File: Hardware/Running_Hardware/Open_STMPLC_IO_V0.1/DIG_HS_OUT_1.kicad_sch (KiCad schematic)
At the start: 25 parts, among them J1 Screw_Terminal_01x02, Q1 SUD50P06, Q2 AO3400A, U7 TPS26600PWP, U8 UCC23513

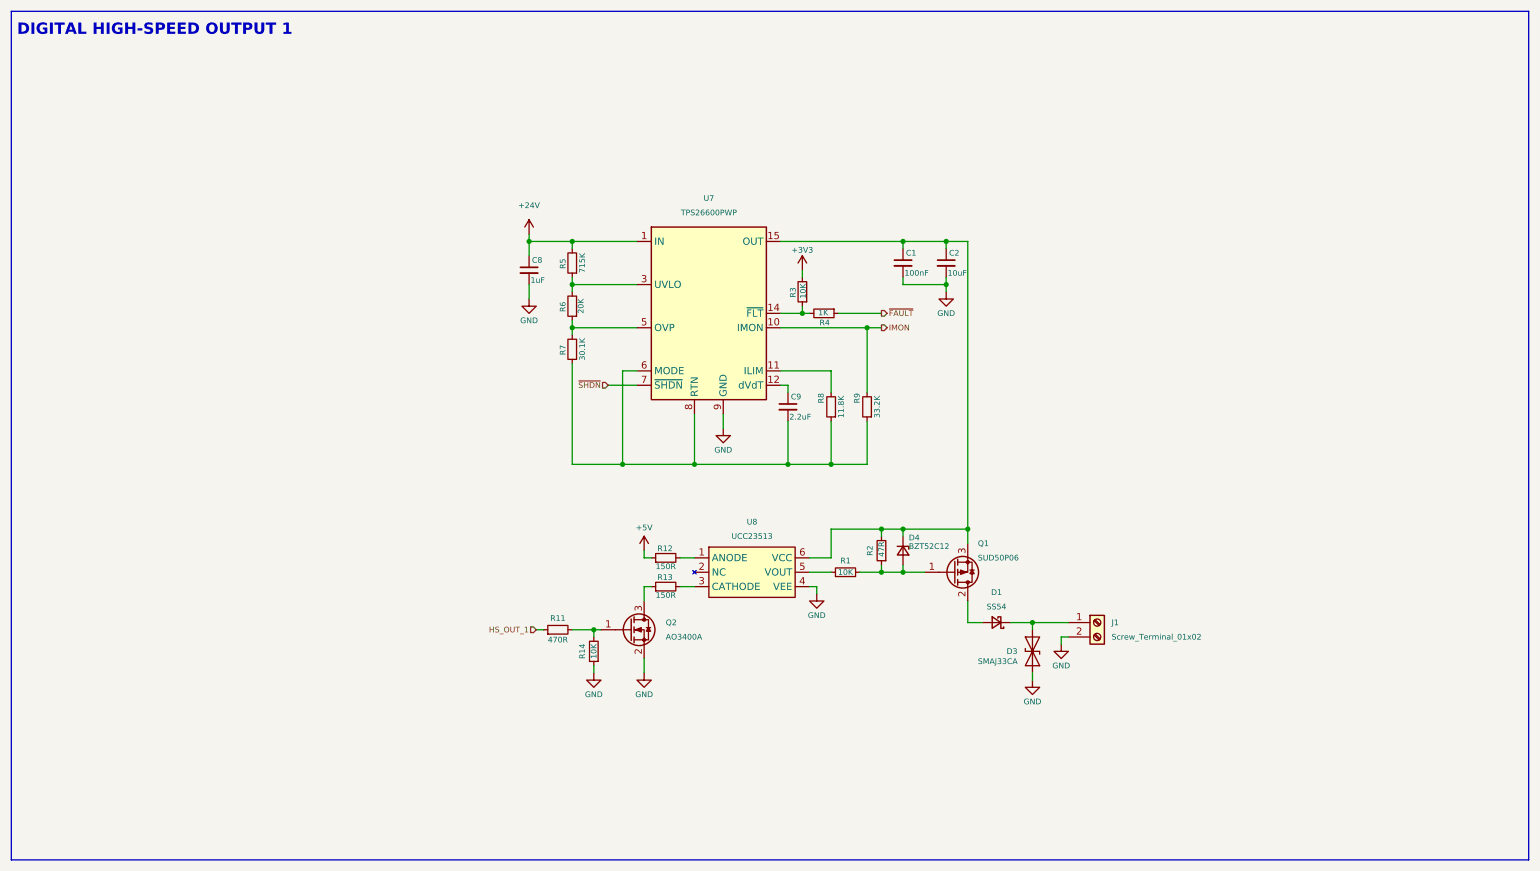
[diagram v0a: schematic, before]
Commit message: Digital IO completion
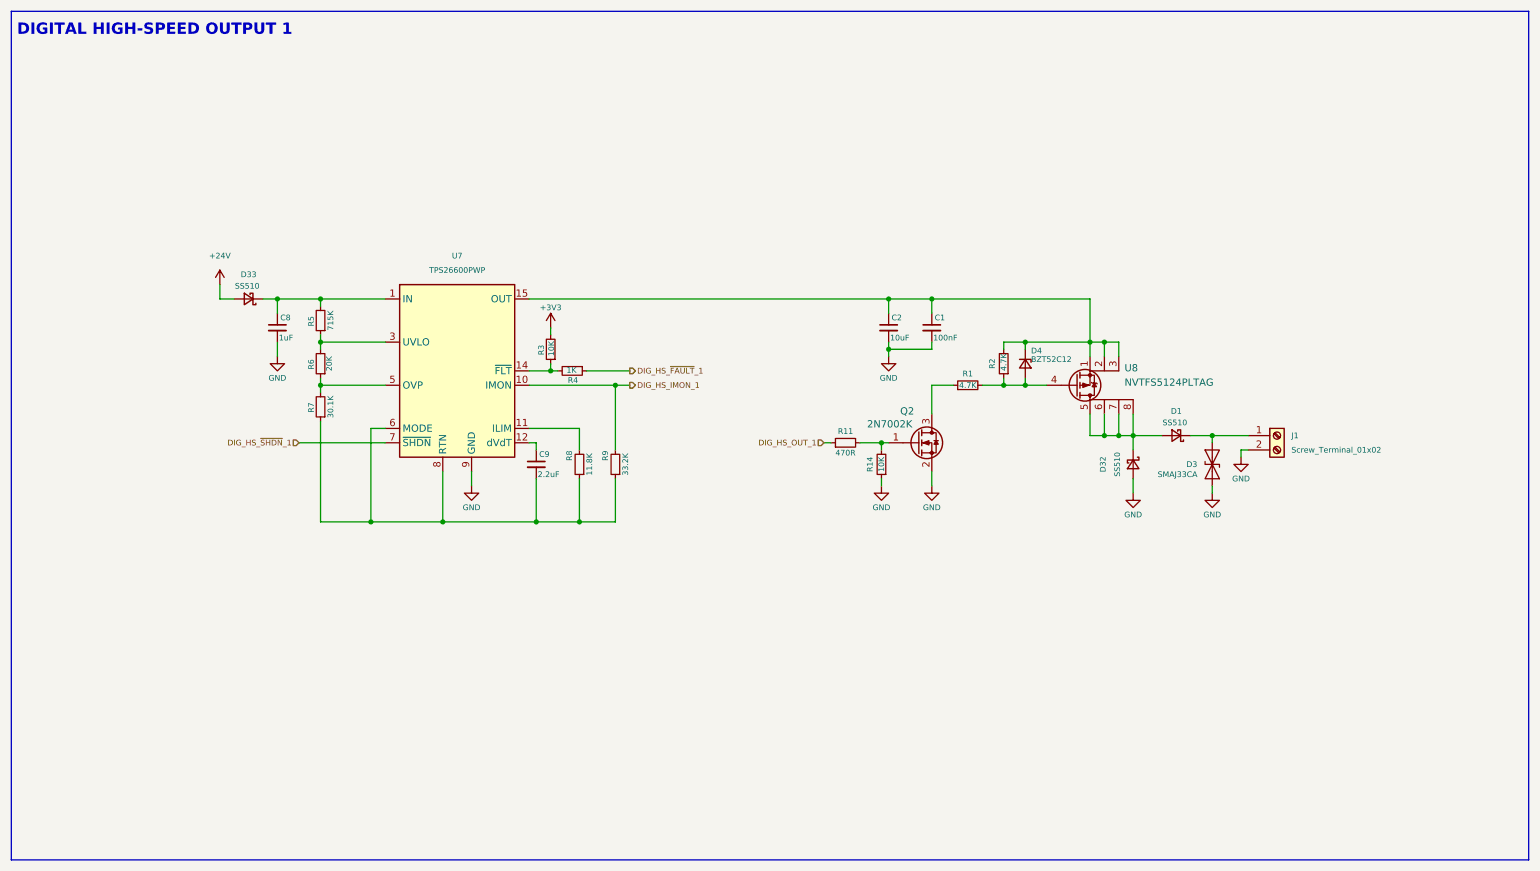
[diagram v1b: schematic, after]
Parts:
- removed Q1: SUD50P06, Package_TO_SOT_SMD:TO-252-3_TabPin2, symbol Transistor_FET:Q_PMOS_GDS
- removed Q2: AO3400A, Package_TO_SOT_SMD:SOT-23, symbol Transistor_FET:AO3400A
- removed R12, R13: 150R, Resistor_SMD:R_0603_1608Metric_Pad0.98x0.95mm_HandSolder, symbol Device:R_Small
- removed U8: UCC23513, Package_SO:SSO-6_6.8x4.6mm_P1.27mm_Clearance8mm, symbol UCC23153:UCC23513
- added D32, D33: SS510, Diode_SMD:D_SMA, symbol Device:D_Schottky_Small
- added Q2: 2N7002K, Package_TO_SOT_SMD:SOT-23, symbol Transistor_FET:2N7002K
- added U8: NVTFS5124PLTAG, NVTFS5124PLTAG:WDFN-8_3.3X3.3_P0.65mm, symbol MOSFET:NVTFS5124PLTAG
- D1: value SS54 -> SS510; footprint (none) -> Diode_SMD:D_SMA
- R1: value 10K -> 4.7K
- R2: value 47R -> 4.7K
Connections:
- net +24V: now also D33.2 (A); no longer C8.1, R5.2, U7.1 (IN), U7.2 (IN)
- net GND: now also D32.2 (A), Q2.2 (S)
- net at C1.1, C2.1, D4.1 (K)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: now also U8.1 (S), U8.2 (S), U8.3 (S)
- net at R11.2, R14.2: now also Q2.1 (G)
- net at D4.2 (A), R1.2, R2.1: now also U8.4 (G)
- net at R1.1: now also Q2.3 (D)
- net at D1.2 (A): now also D32.1 (K), U8.5, U8.6 (D), U8.7 (D), U8.8 (D)
- net HS_OUT_1 renamed DIG_HS_OUT_1
- net IMON renamed DIG_HS_IMON_1
- net ~{FAULT} renamed DIG_HS_~{FAULT}_1
- net ~{SHDN} renamed DIG_HS_~{SHDN}_1
- new net: C8.1, D33.1 (K), R5.2, U7.1 (IN), U7.2 (IN)
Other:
- moved on the sheet: C1, C2, C8, C9, D1, D3, D4, J1, R1, R11, R14, R2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

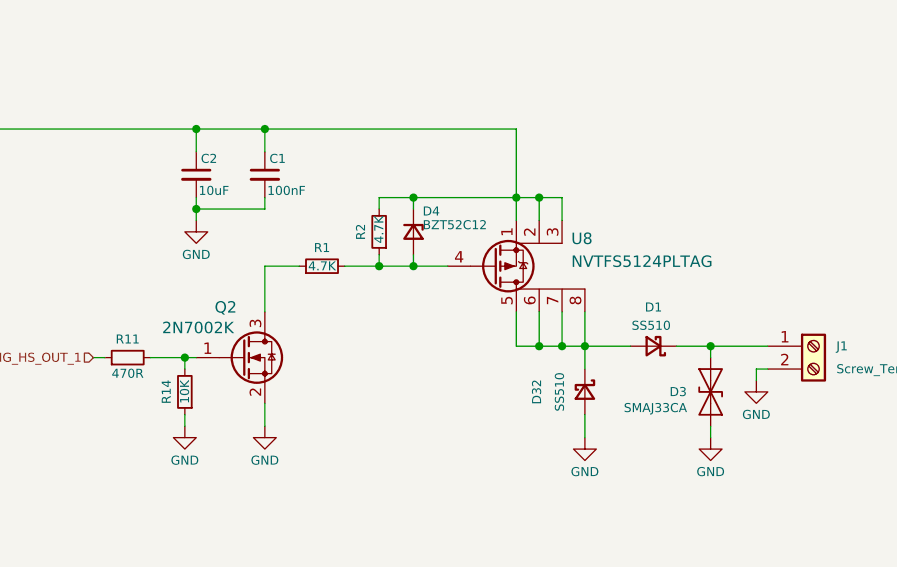
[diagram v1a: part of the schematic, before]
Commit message: Analog input section
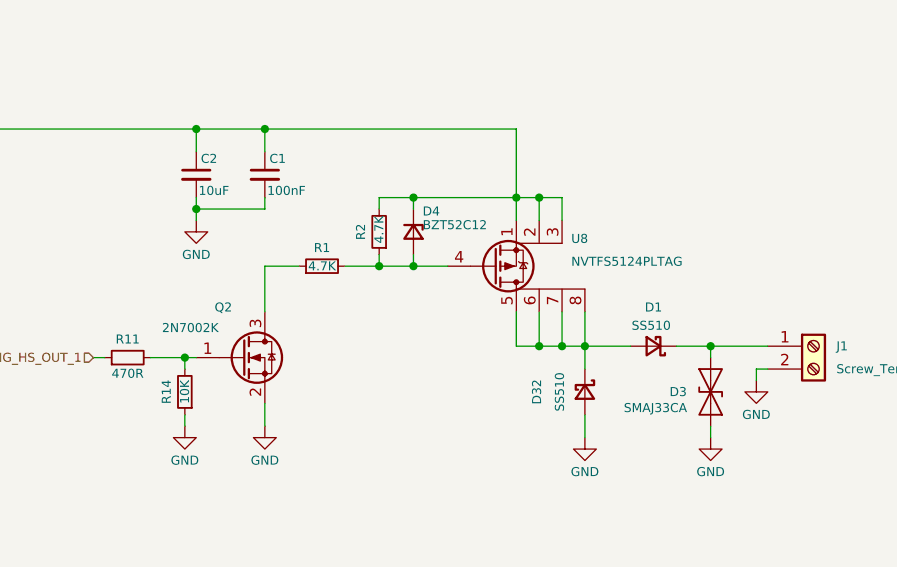
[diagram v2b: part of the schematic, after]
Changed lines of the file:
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@@
 			(effects
 				(font
-					(size 1.27 1.27)
+					(size 1 1)
 				)
 				(justify left)
@@
 			(effects
 				(font
-					(size 1.27 1.27)
+					(size 1 1)
 				)
 				(justify left)
@@
 			(effects
 				(font
-					(size 1.27 1.27)
+					(size 1 1)
 				)
 				(justify left)
@@
 			(effects
 				(font
-					(size 1.27 1.27)
+					(size 1 1)
 				)
 				(justify left)
